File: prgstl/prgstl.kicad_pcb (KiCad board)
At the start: 2 copper layers, 76.2 x 50.8 mm, 49 parts, among them J2 STM32WORLD_BASE, Q1 S9013, U1 AMS1117-3.3, U2 STM32F103CBTx, U3 SRV05-4, Y1 X_8MHZ

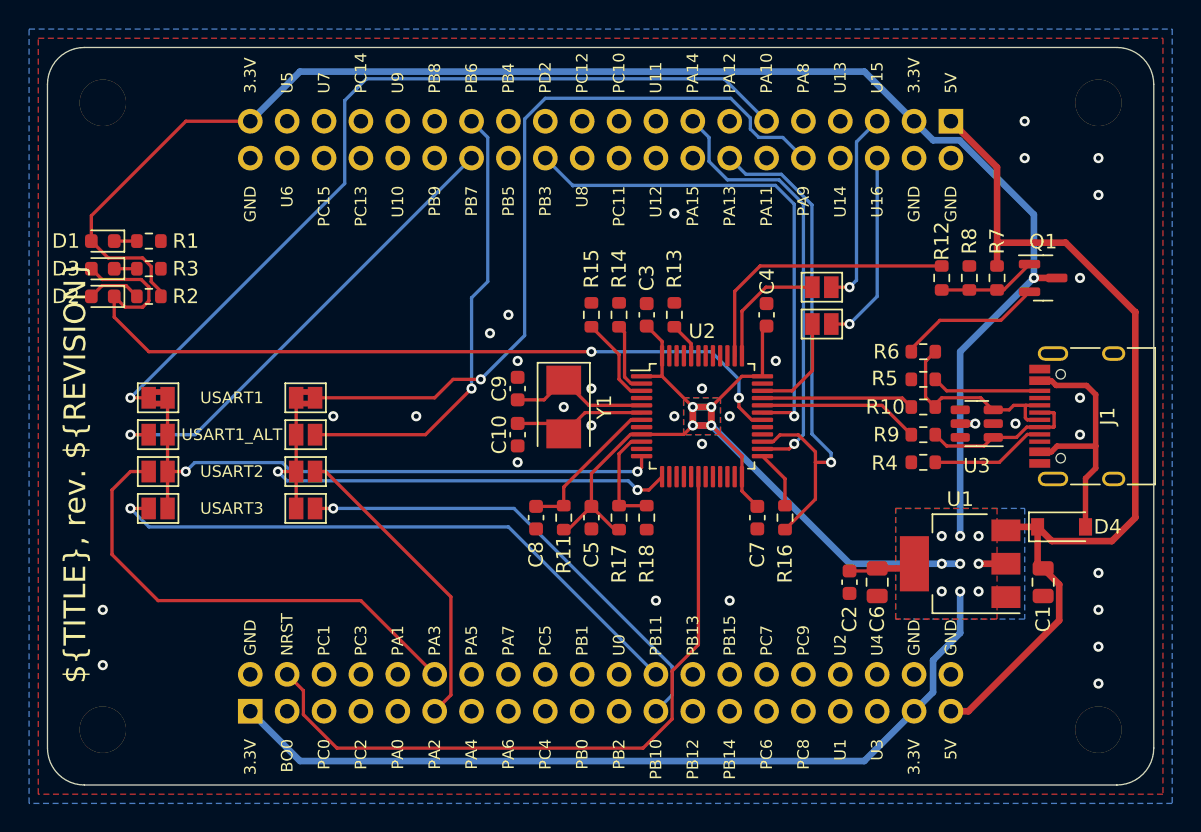
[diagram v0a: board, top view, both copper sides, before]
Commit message: Hmmmm
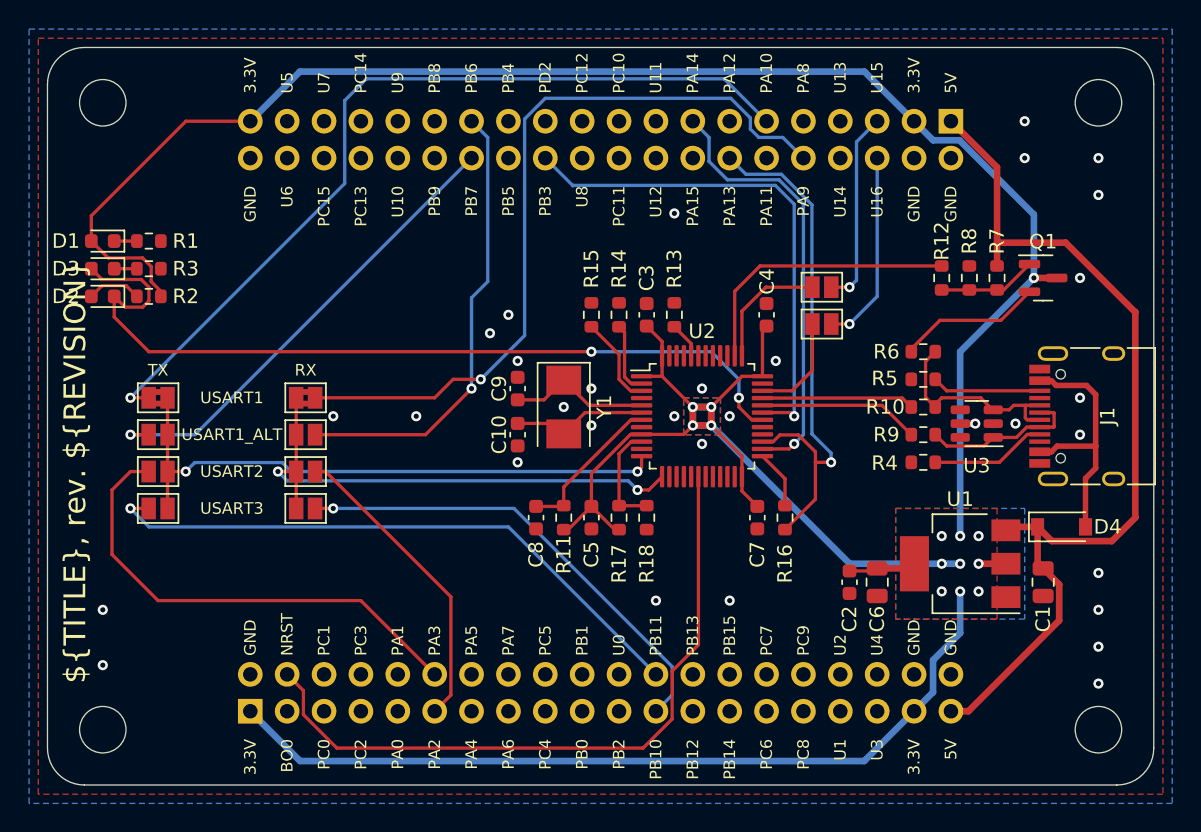
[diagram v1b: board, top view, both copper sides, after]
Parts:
- U1: value AMS1117-3.3 -> AMS1117-3.3``
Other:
- board text added: "RX"
- board text added: "TX"

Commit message: Hmmm
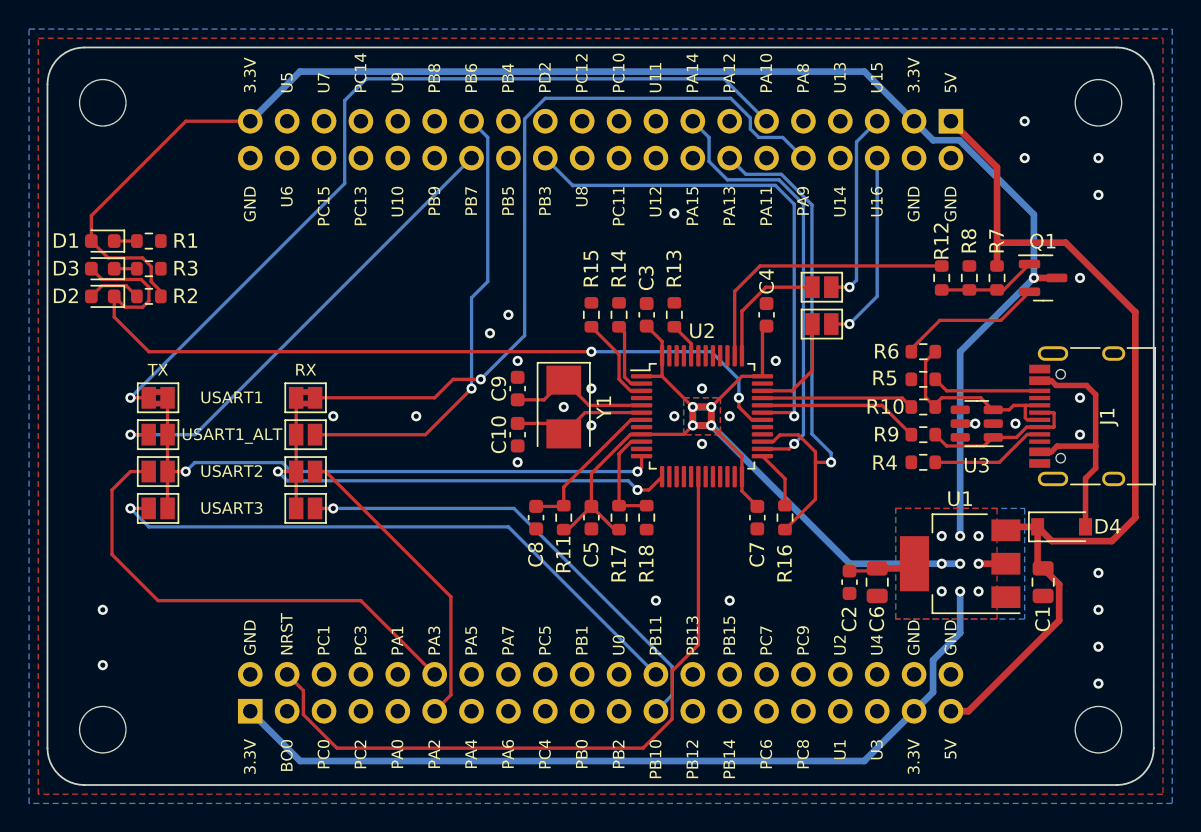
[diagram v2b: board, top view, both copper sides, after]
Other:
- board text removed: "${TITLE}, rev. ${REVISION}"

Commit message: Playing with ordering files
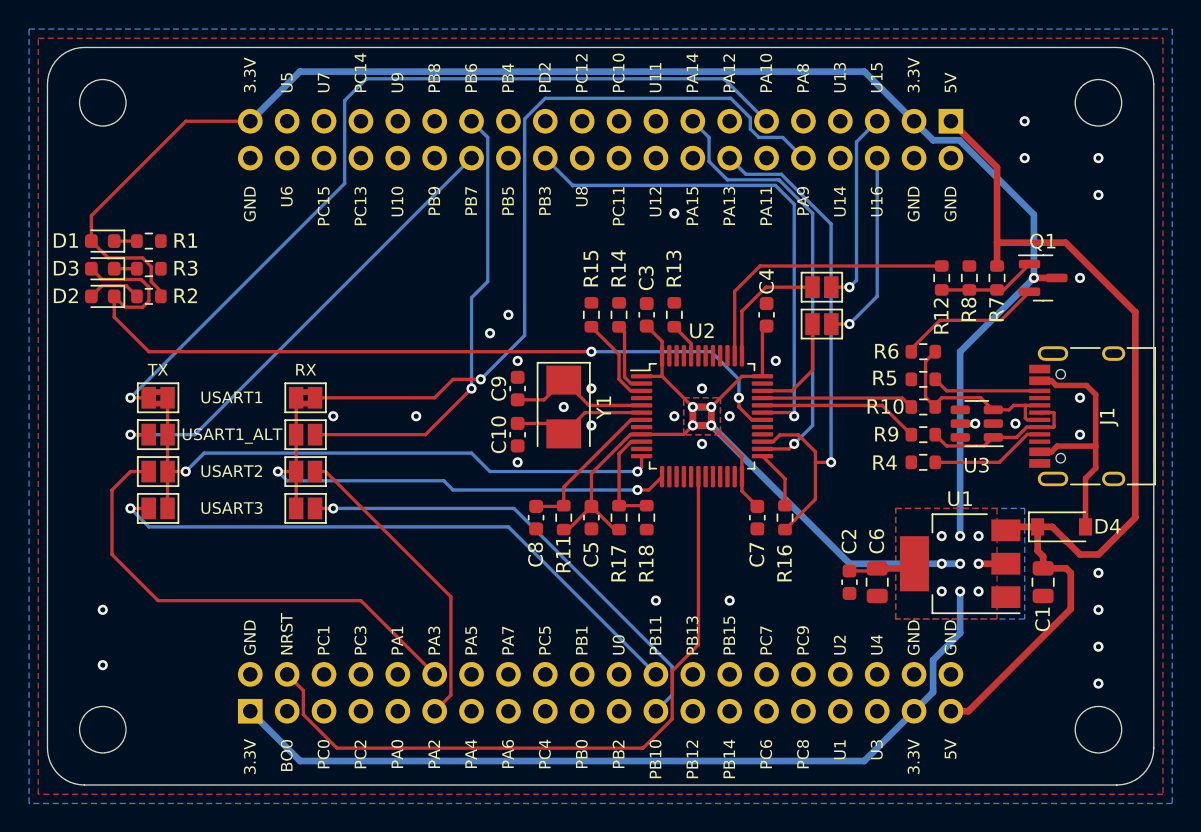
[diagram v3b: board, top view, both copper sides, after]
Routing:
- net +5V: track 63.8 -> 66.2 mm
- net T_TX: track 41.7 -> 42.2 mm
- net T_CLK: track 30.1 -> 30.6 mm

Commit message: Hmmm
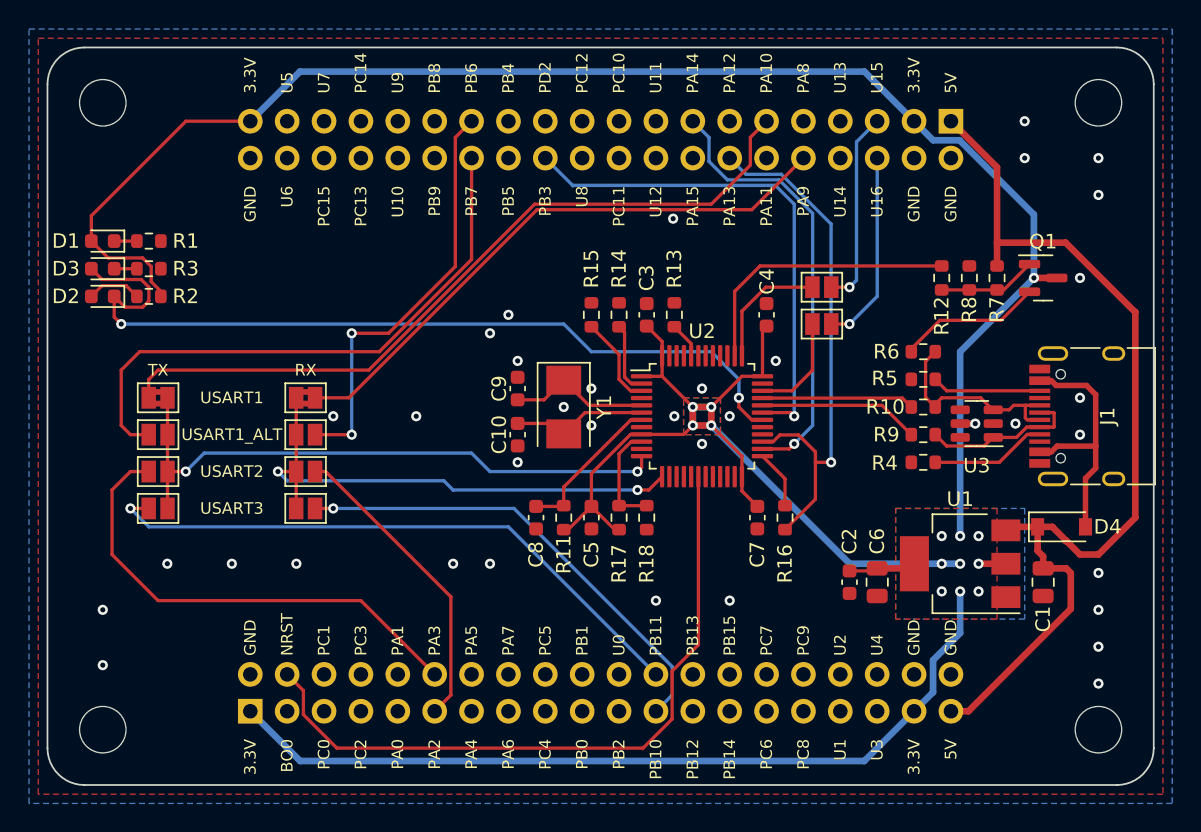
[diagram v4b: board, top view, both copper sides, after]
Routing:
- net USART1_TX: track 53.1 -> 40.5 mm, vias 1 -> 0
- net USART1_RX_ALT: track 32.6 -> 40.2 mm, vias 1 -> 0
- net USART1_RX: track 58.7 -> 52.3 mm, vias 1 -> 0
- net USART1_TX_ALT: track 31.4 -> 29.0 mm, vias 1 -> 2
- net GND: vias 31 -> 36
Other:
- board text added: "JLCJLCJLCJLC"

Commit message: Hmmmm
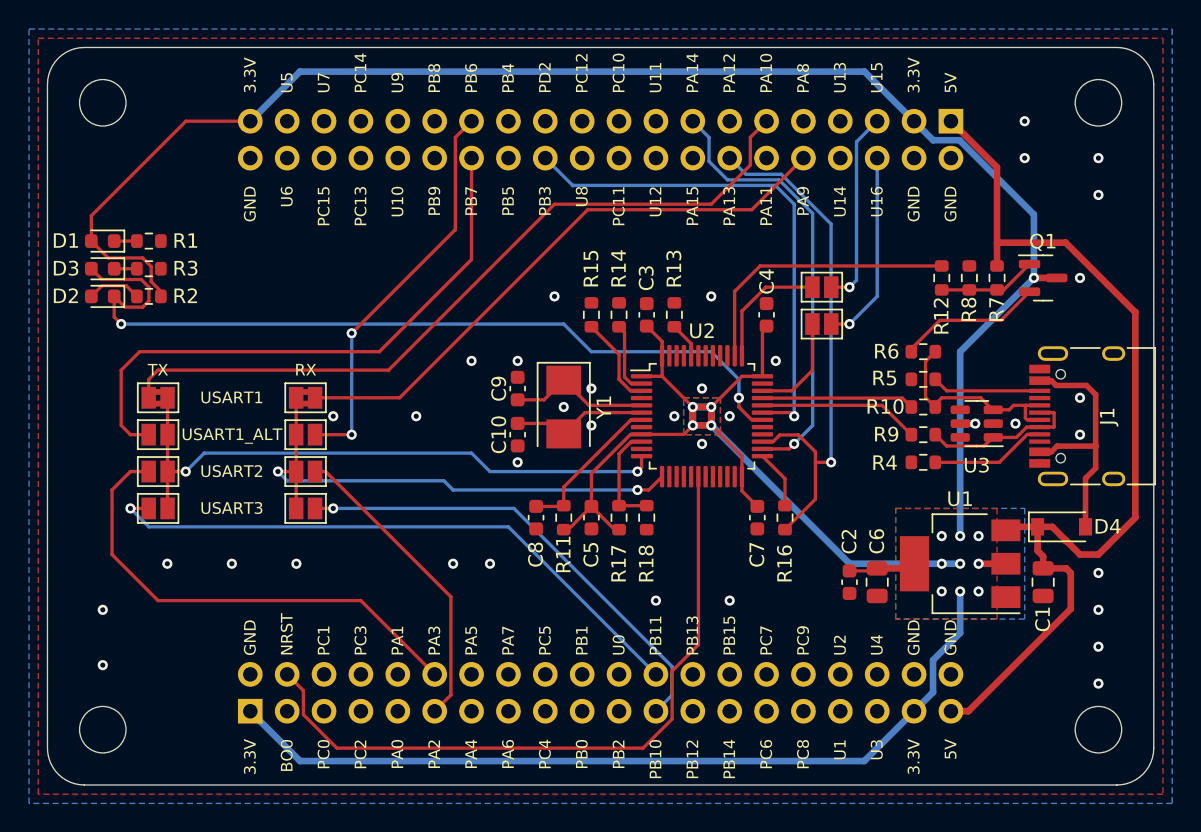
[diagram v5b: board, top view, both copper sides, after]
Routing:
- net USART1_TX_ALT: track 29.0 -> 27.5 mm
